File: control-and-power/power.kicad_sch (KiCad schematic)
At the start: 1 part

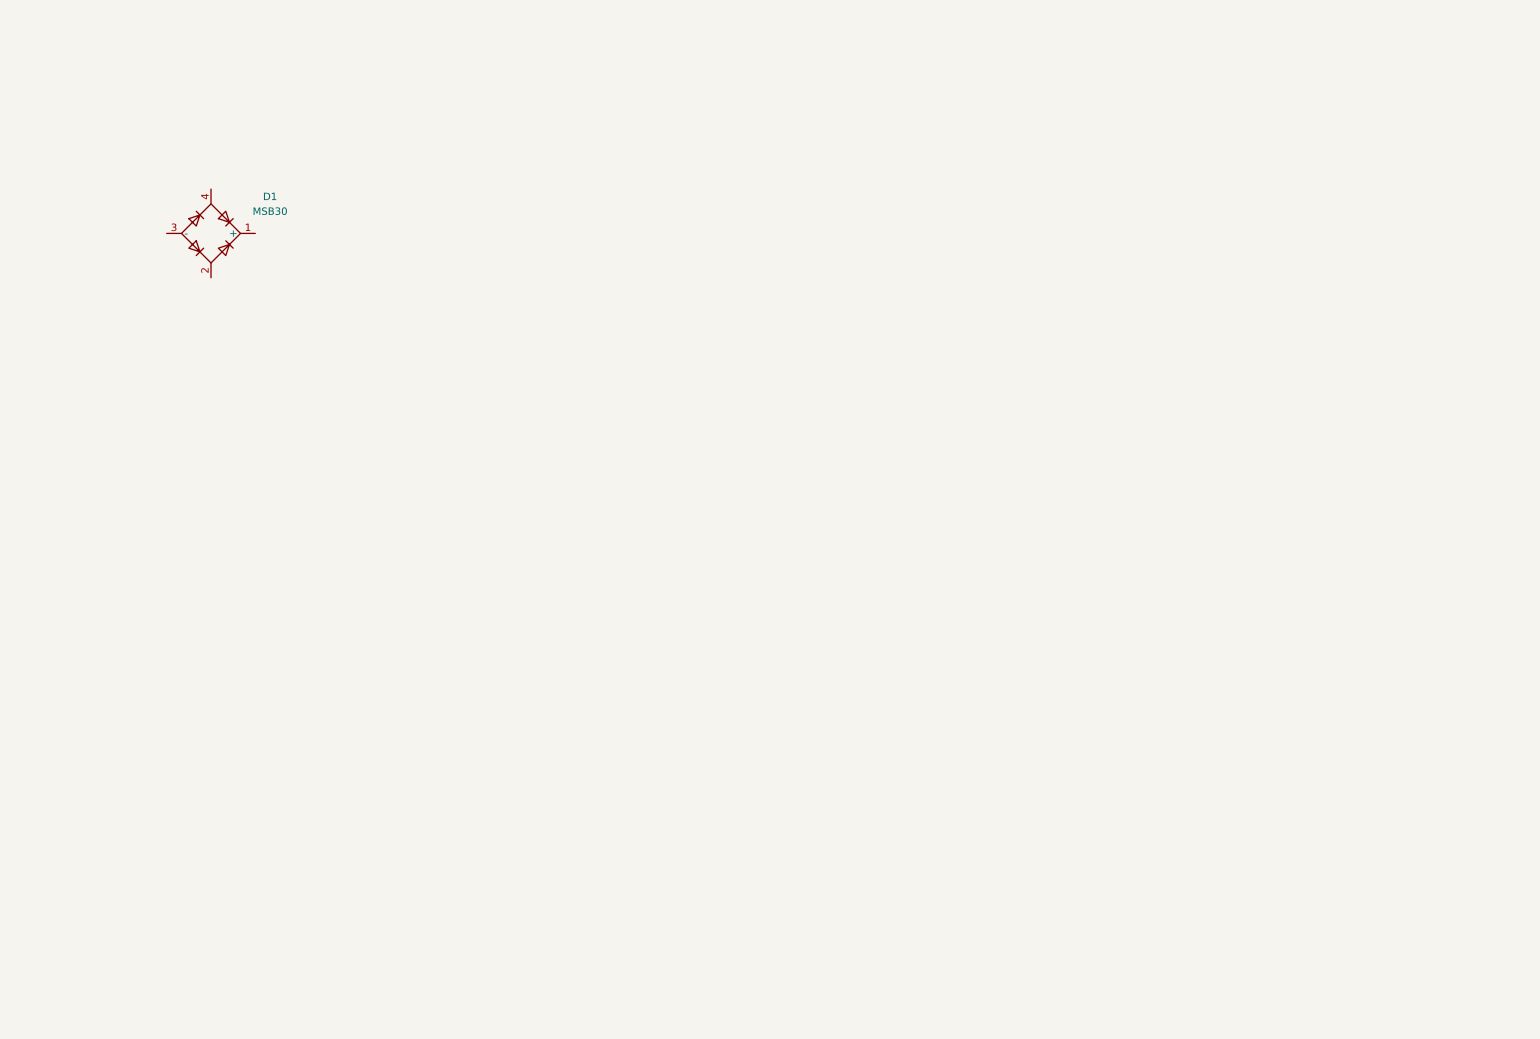
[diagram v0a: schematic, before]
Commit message: 15
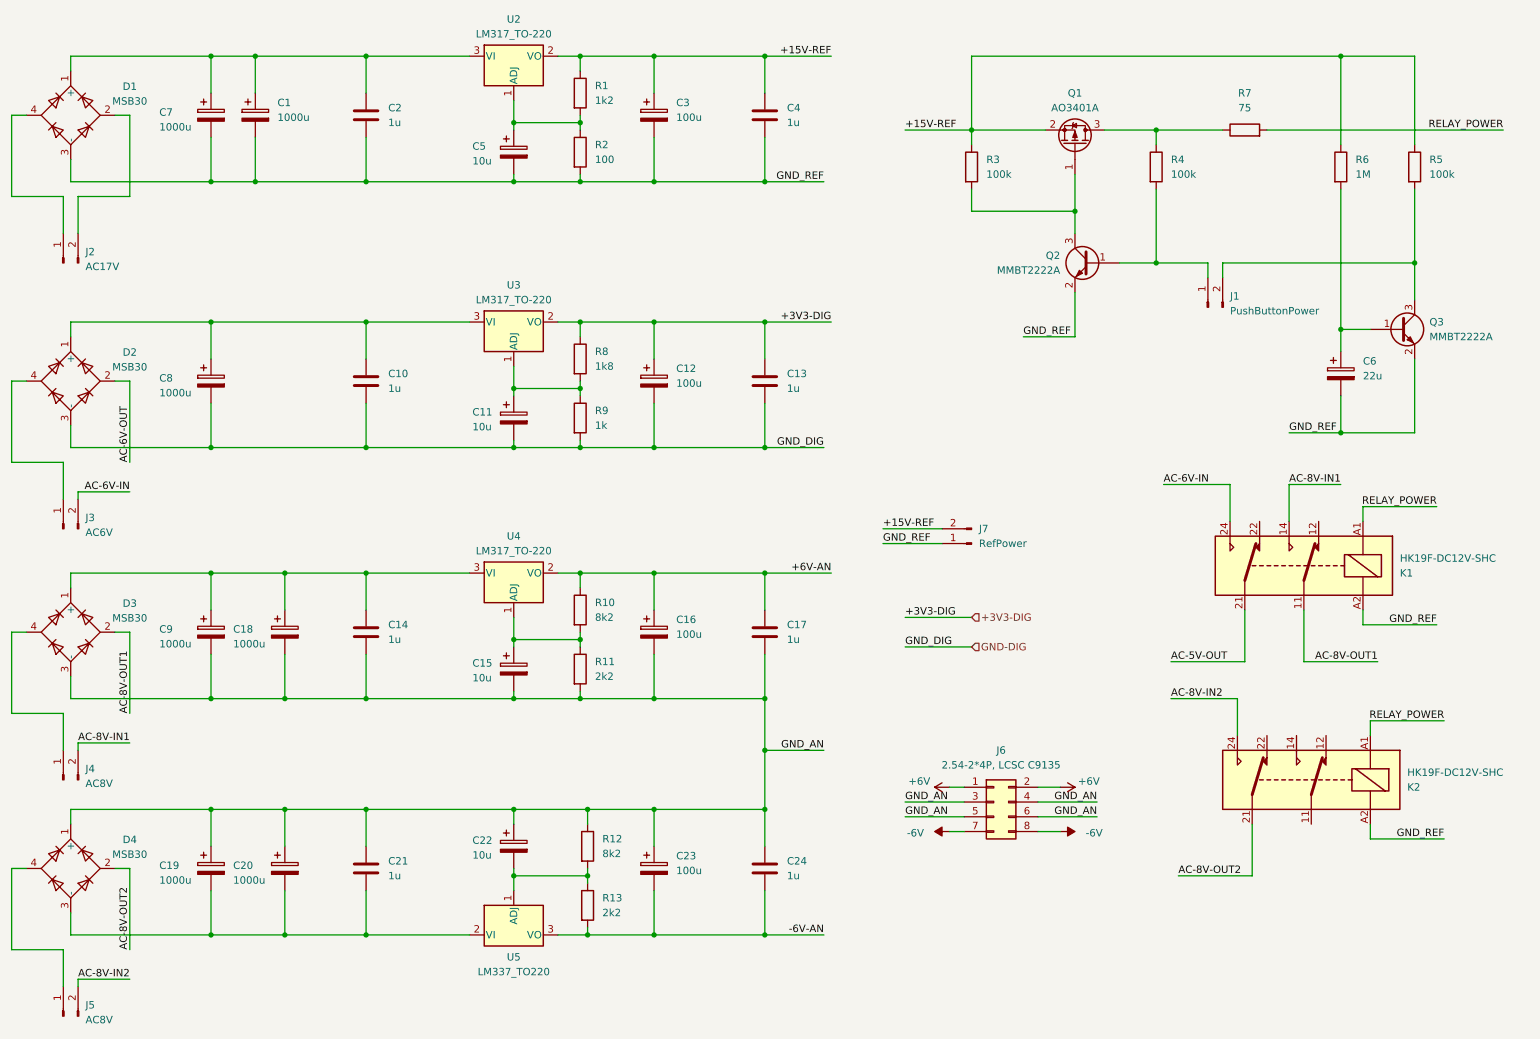
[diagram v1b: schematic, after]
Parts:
- added C1, C18, C19, C20, C7, C8, C9: 1000u, Capacitor_SMD:CP_Elec_CAP-XX_DMF3Zxxxxxxxx3D, symbol Device:C_Polarized
- added C10, C13, C14, C17, C2, C21, C24, C4: 1u, Capacitor_SMD:C_0805_2012Metric_Pad1.18x1.45mm_HandSolder, symbol Device:C
- added C11, C15, C22, C5: 10u, Capacitor_SMD:CP_Elec_CAP-XX_DMF3Zxxxxxxxx3D, symbol Device:C_Polarized
- added C12, C16, C23, C3: 100u, Capacitor_SMD:CP_Elec_CAP-XX_DMF3Zxxxxxxxx3D, symbol Device:C_Polarized
- added C6: 22u, Capacitor_SMD:CP_Elec_CAP-XX_DMF3Zxxxxxxxx3D, symbol Device:C_Polarized
- added D2, D3, D4: MSB30, Passives:MSB30, symbol Passives:MSB30
- added J1: PushButtonPower, Connector_PinHeader_2.54mm:PinHeader_1x02_P2.54mm_Vertical, symbol Connector:Conn_01x02_Pin
- added J2: AC17V, Connector_PinHeader_2.54mm:PinHeader_1x02_P2.54mm_Vertical, symbol Connector:Conn_01x02_Pin
- added J3: AC6V, Connector_PinHeader_2.54mm:PinHeader_1x02_P2.54mm_Vertical, symbol Connector:Conn_01x02_Pin
- added J4, J5: AC8V, Connector_PinHeader_2.54mm:PinHeader_1x02_P2.54mm_Vertical, symbol Connector:Conn_01x02_Pin
- added J6: 2.54-2*4P, LCSC C9135, Connector_IDC:IDC-Header_2x04_P2.54mm_Vertical, symbol Connector_Generic:Conn_02x04_Odd_Even
- added J7: RefPower, Connector_PinHeader_2.54mm:PinHeader_1x02_P2.54mm_Vertical, symbol Connector:Conn_01x02_Pin
- added K1, K2: HK19F-DC12V-SHC, Relay_THT:Relay_DPDT_Finder_30.22, symbol Relay:HK19F-DCxxV-SHC
- added Q1: AO3401A, Package_TO_SOT_SMD:SOT-23, symbol Transistor_FET:AO3401A
- added Q2, Q3: MMBT2222A, Package_TO_SOT_SMD:SOT-23, symbol Transistor_BJT:MMBT2222A
- added R1: 1k2, Resistor_SMD:R_1206_3216Metric_Pad1.30x1.75mm_HandSolder, symbol Device:R
- added R10, R12: 8k2, Resistor_SMD:R_1206_3216Metric_Pad1.30x1.75mm_HandSolder, symbol Device:R
- added R11, R13: 2k2, Resistor_SMD:R_1206_3216Metric_Pad1.30x1.75mm_HandSolder, symbol Device:R
- added R2: 100, Resistor_SMD:R_1206_3216Metric_Pad1.30x1.75mm_HandSolder, symbol Device:R
- added R3, R4, R5: 100k, Resistor_SMD:R_1206_3216Metric_Pad1.30x1.75mm_HandSolder, symbol Device:R
- added R6: 1M, Resistor_SMD:R_1206_3216Metric_Pad1.30x1.75mm_HandSolder, symbol Device:R
- added R7: 75, Resistor_SMD:R_1206_3216Metric_Pad1.30x1.75mm_HandSolder, symbol Device:R
- added R8: 1k8, Resistor_SMD:R_1206_3216Metric_Pad1.30x1.75mm_HandSolder, symbol Device:R
- added R9: 1k, Resistor_SMD:R_1206_3216Metric_Pad1.30x1.75mm_HandSolder, symbol Device:R
- added U2, U3, U4: LM317_TO-220, Package_TO_SOT_THT:TO-220-3_Vertical, symbol Regulator_Linear:LM317_TO-220
- added U5: LM337_TO220, Package_TO_SOT_THT:TO-220-3_Vertical, symbol Regulator_Linear:LM337_TO220
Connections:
- net at D1.1 (+): now also C1.1, C2.1, C7.1, U2.3 (VI)
- net at D1.2: now also J2.2 (Pin_2)
- net GND_REF: now reaches D1.3 (-)
- net GND_REF: now also C1.2, C2.2, C3.2, C4.2, C5.2, C6.2, C7.2, J7.1 (Pin_1), K1.A2, K2.A2, Q2.2 (E), Q3.2 (E), R2.2
- net at D1.4: now also J2.1 (Pin_1)
- new net: D2.4, J3.1 (Pin_1)
- new net: C11.1, R8.2, R9.1, U3.1 (ADJ)
- new net: Q1.1 (G), Q2.3 (C), R3.2
- new net: C19.2, C20.2, C21.2, D4.3 (-), U5.2 (VI)
- new net: D4.4, J5.1 (Pin_1)
- new net: C22.2, R12.2, R13.1, U5.1 (ADJ)
- new net: C6.1, Q3.1 (B), R6.2
- new net: Q1.3 (D), R4.1, R7.1
- new net: J1.1 (Pin_1), Q2.1 (B), R4.2
- new net: C5.1, R1.2, R2.1, U2.1 (ADJ)
- new net: C10.1, C8.1, D2.1 (+), U3.3 (VI)
- new net: C14.1, C18.1, C9.1, D3.1 (+), U4.3 (VI)
- new net: J1.2 (Pin_2), Q3.3 (C), R5.2
- new net: C15.1, R10.2, R11.1, U4.1 (ADJ)
- new net: D3.4, J4.1 (Pin_1)
- new net +15V-REF: C3.1, C4.1, J7.2 (Pin_2), Q1.2 (S), R1.1, R3.1, R5.1, R6.1, U2.2 (VO)
- new net +3V3-DIG: C12.1, C13.1, R8.1, U3.2 (VO)
- new net +6V: J6.1 (Pin_1), J6.2 (Pin_2)
- new net +6V-AN: C16.1, C17.1, R10.1, U4.2 (VO)
- new net -6V: J6.7 (Pin_7), J6.8 (Pin_8)
- new net -6V-AN: C23.2, C24.2, R13.2, U5.3 (VO)
- new net AC-5V-OUT: K1.21
- new net AC-6V-IN: J3.2 (Pin_2), K1.24
- new net AC-6V-OUT: D2.2
- new net AC-8V-IN1: J4.2 (Pin_2), K1.14
- new net AC-8V-IN2: J5.2 (Pin_2), K2.24
- new net AC-8V-OUT1: D3.2, K1.11
- new net AC-8V-OUT2: D4.2, K2.21
- new net GND-DIG: C10.2, C11.2, C12.2, C13.2, C8.2, D2.3 (-), R9.2
- new net GND_AN: C14.2, C15.2, C16.2, C17.2, C18.2, C19.1, C20.1, C21.1, C22.1, C23.1, C24.1, C9.2, D3.3 (-), D4.1 (+), J6.3 (Pin_3), J6.4 (Pin_4), J6.5 (Pin_5), J6.6 (Pin_6), R11.2, R12.1
- new net RELAY_POWER: K1.A1, K2.A1, R7.2
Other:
- moved on the sheet: D1

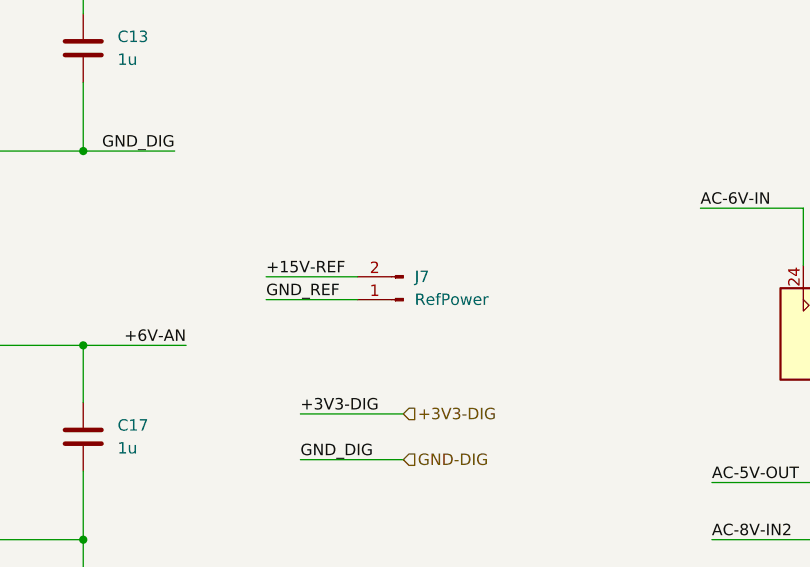
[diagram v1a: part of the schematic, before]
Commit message: 16
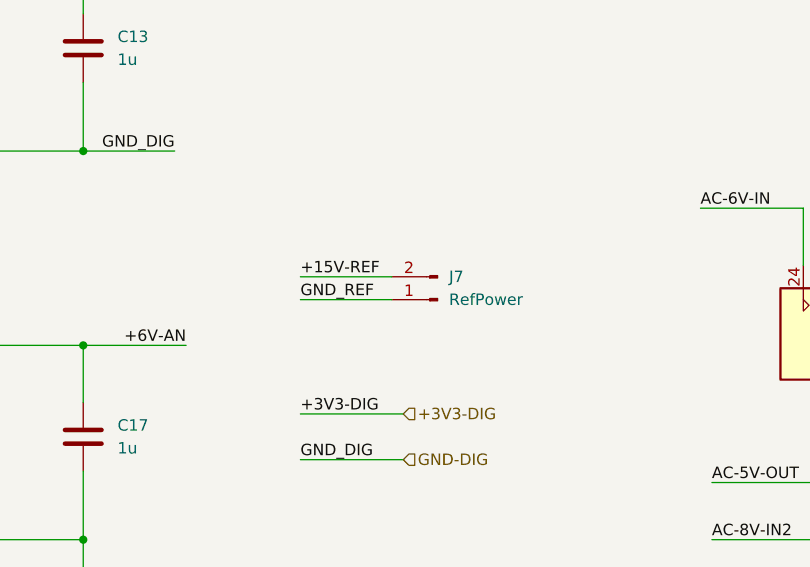
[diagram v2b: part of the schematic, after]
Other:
- moved on the sheet: J7
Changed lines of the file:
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@@
 	(wire
 		(pts
-			(xy 172.72 106.68) (xy 182.88 106.68)
+			(xy 176.53 106.68) (xy 186.69 106.68)
 		)
 		(stroke
@@
 	(wire
 		(pts
-			(xy 172.72 104.14) (xy 182.88 104.14)
+			(xy 176.53 104.14) (xy 186.69 104.14)
 		)
 		(stroke
@@
 	)
 	(label "GND_REF"
-		(at 172.72 106.68 0)
+		(at 176.53 106.68 0)
 		(effects
 			(font
@@
 	)
 	(label "+15V-REF"
-		(at 172.72 104.14 0)
+		(at 176.53 104.14 0)
 		(effects
 			(font
@@
 	(symbol
 		(lib_id "Connector:Conn_01x02_Pin")
-		(at 187.96 106.68 180)
+		(at 191.77 106.68 180)
 		(unit 1)
 		(exclude_from_sim no)
@@
 		(fields_autoplaced yes)
 		(property "Reference" "J7"
-			(at 189.23 104.1399 0)
+			(at 193.04 104.1399 0)
 			(effects
 				(font
@@
 		)
 		(property "Value" "RefPower"
-			(at 189.23 106.6799 0)
+			(at 193.04 106.6799 0)
 			(effects
 				(font
@@
 		)
 		(property "Footprint" "Connector_PinHeader_2.54mm:PinHeader_1x02_P2.54mm_Vertical"
-			(at 187.96 106.68 0)
+			(at 191.77 106.68 0)
 			(effects
 				(font
@@
 		)
 		(property "Datasheet" "~"
-			(at 187.96 106.68 0)
+			(at 191.77 106.68 0)
 			(effects
 				(font
@@
 		)
 		(property "Description" "Generic connector, single row, 01x02, script generated"
-			(at 187.96 106.68 0)
+			(at 191.77 106.68 0)
 			(effects
 				(font
